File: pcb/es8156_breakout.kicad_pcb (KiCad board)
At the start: 2 copper layers, 24.4 x 31.5 mm, 9 parts, among them CN1 PJ-320D, J2 Conn_01x12, J3 Conn_01x03, U1 ES8156

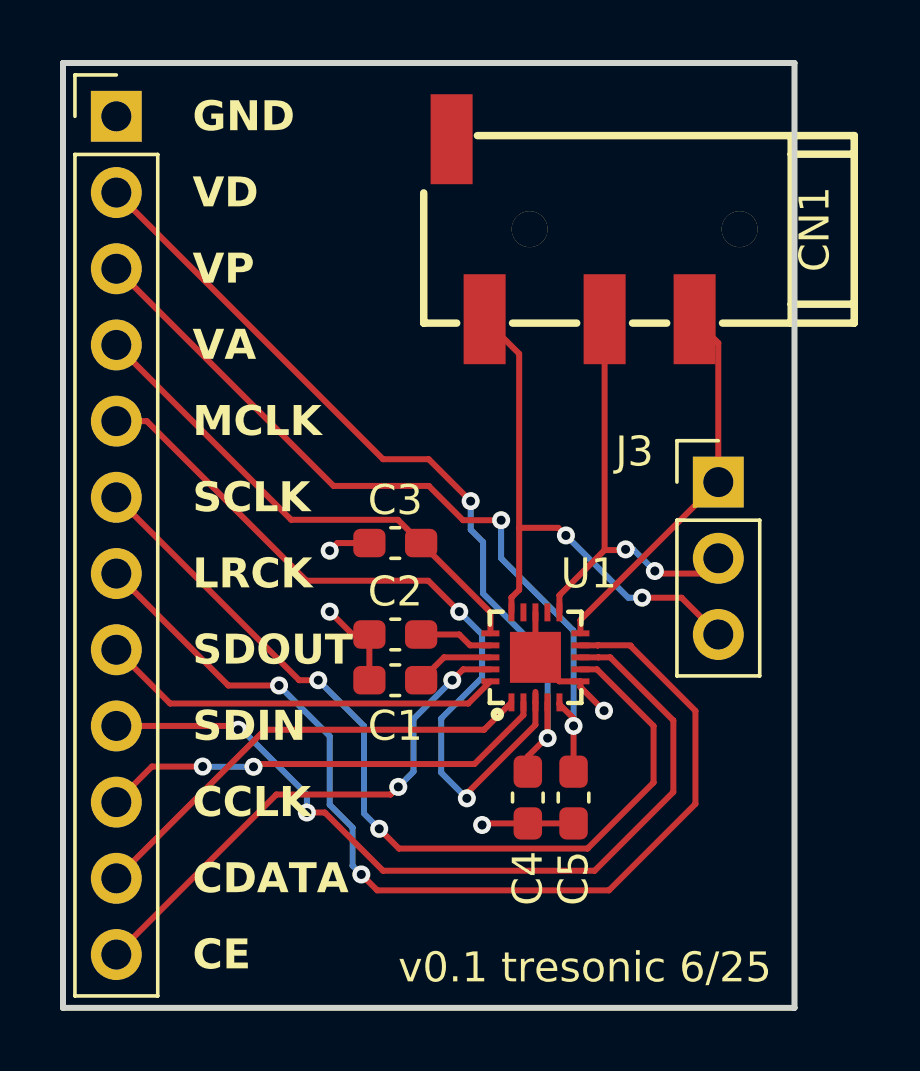
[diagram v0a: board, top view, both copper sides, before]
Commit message: update schematic & pcb
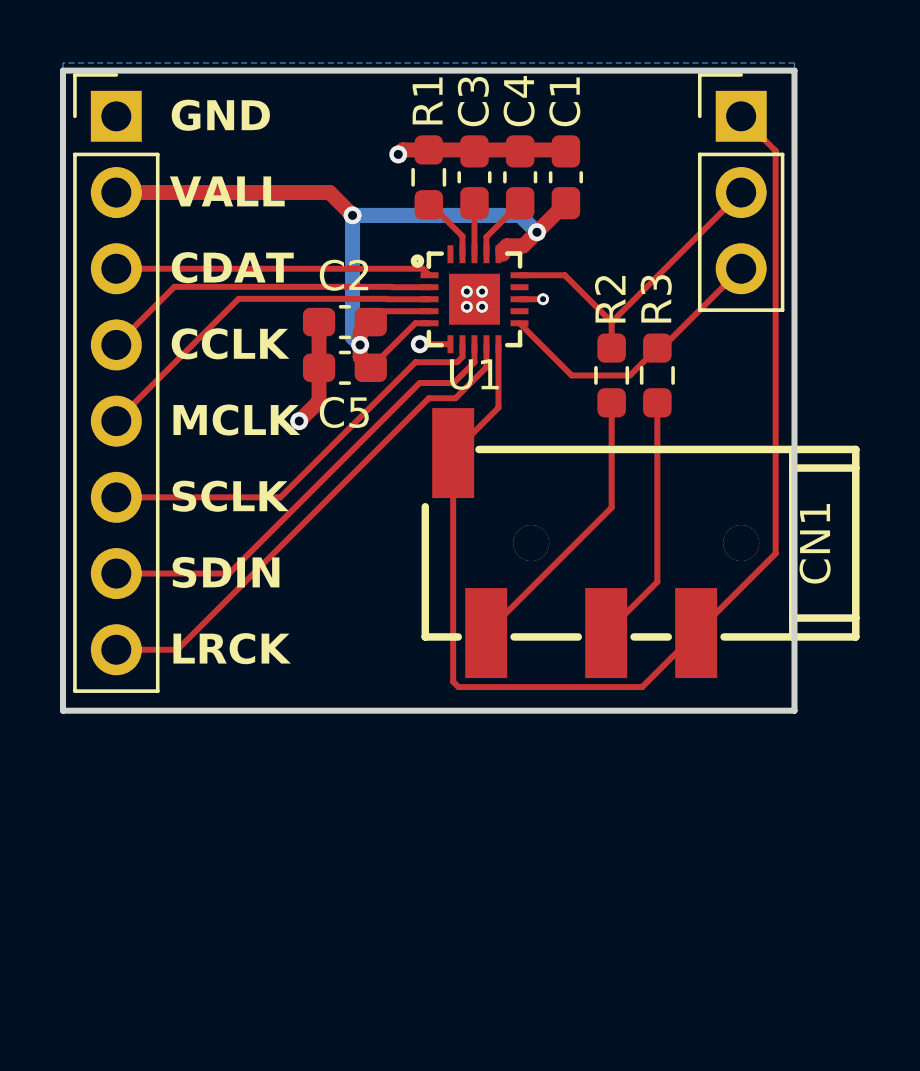
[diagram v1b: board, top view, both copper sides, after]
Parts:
- removed the J2 at (25.1, 24.7)
- added J1: Conn_01x08, Connector_PinHeader_2.54mm:PinHeader_1x08_P2.54mm_Vertical, F.Cu at (25.1, 24.7)
- added R1: 10k, Resistor_SMD:R_0603_1608Metric_Pad0.98x0.95mm_HandSolder, F.Cu at (35.5, 26.8)
- added R2: 33R, Resistor_SMD:R_0603_1608Metric_Pad0.98x0.95mm_HandSolder, F.Cu at (41.6, 33.4)
- added R3: 33R, Resistor_SMD:R_0603_1608Metric_Pad0.98x0.95mm_HandSolder, F.Cu at (43.2, 33.4)
- C5: value 100n -> 1u
- moved C4 20.7 mm to (38.6, 26.8)
- moved C1 17.7 mm to (40.1, 26.8), turned to 90 degrees
- moved C5 16.2 mm to (32.7, 33.1), turned to 0 degrees
- moved C3 12.5 mm to (37.1, 26.8), turned to -90 degrees
- moved J2 12.2 mm to (46.0, 24.7)
- moved U1 12.1 mm to (37.1, 30.8), turned to 0 degrees
- moved C2 10.5 mm to (32.7, 31.6), turned to 180 degrees
- moved CN1 10.5 mm to (40.4, 38.9)
- renumbered J3 to J2
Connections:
- C1 pad 1: GND -> VALL
- C1 pad 2: Net-(U1-VMID) -> GND
- C2 pad 1: GND -> VALL
- C2 pad 2: Net-(U1-VRP) -> GND
- C3 pad 2: VA -> Net-(U1-VMID)
- C4 pad 1: VD -> GND
- C4 pad 2: GND -> Net-(U1-VRP)
- C5 pad 1: VP -> GND
- C5 pad 2: GND -> VALL
- CN1 pad 1: unconnected-(CN1-Pad1) -> /HPCOM
- CN1 pad 3: /Right -> /HP_Right
- CN1 pad 4: /Left -> /HP_Left
- J2 pad 2: /Right -> /Left
- J2 pad 3: /Left -> /Right
- U1 pad 16: VA -> VALL
- U1 pad 19: /CE -> Net-(U1-CE)
- U1 pad 20: /SDOUT -> unconnected-(U1-SDOUT-Pad20)
- U1 pad 4: VD -> VALL
- U1 pad 5: VP -> VALL
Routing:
- net VALL: track 0.00 -> 28.4 mm, vias 0 -> 3
- net VD: track 27.7 -> 0.00 mm, vias 2 -> 0
- net /HPCOM: track 12.7 -> 39.8 mm
- net VP: track 26.7 -> 0.00 mm, vias 2 -> 0
- net /LRCK: track 34.8 -> 17.0 mm, vias 2 -> 0
- net /CE: track 17.4 -> 0.00 mm, vias 2 -> 0
- net VA: track 16.9 -> 0.00 mm
- net /SCLK: track 30.5 -> 13.9 mm, vias 2 -> 0
- net /MCLK: track 26.0 -> 12.1 mm, vias 2 -> 0
- net /SDOUT: track 13.5 -> 0.00 mm
- net /SDIN: track 28.4 -> 15.5 mm, vias 2 -> 0
- net /HP_Left: track 0.00 -> 9.41 mm
- net /HP_Right: track 0.00 -> 8.38 mm
- net /Left: track 18.5 -> 10.7 mm, vias 2 -> 0
- net /Right: track 14.7 -> 9.58 mm, vias 2 -> 0
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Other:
- board size 24.4 x 31.5 mm -> 24.4 x 21.3 mm
- board text added: "CDAT"
- board text added: "VALL"
- board text removed: "CDATA"
- board text removed: "CE"
- board text removed: "SDOUT"
- board text removed: "VA"
- board text removed: "VD"
- board text removed: "VP"
- board text removed: "v0.1 tresonic 6/25"
